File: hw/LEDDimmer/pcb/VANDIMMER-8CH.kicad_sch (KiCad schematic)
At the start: 42 parts, among them J1 PWR_IN, J10 BTN1, J11 BTN2, J2 CH1, J3 CH2, J4 CH3, J5 CH4, J6 CH5, J7 CH6, J8 CH7, J9 CH8, Q1 IRLZ44N, Q2 IRLZ44N, Q3 IRLZ44N, Q4 IRLZ44N, Q5 IRLZ44N, Q6 IRLZ44N, Q7 IRLZ44N, Q8 IRLZ44N, U1 LM1117T-3.3, U2 ESP32-DevkitC-1

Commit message: hw
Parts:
- J2, J3, J4, J5, J6, J7, J8, J9: footprint TerminalBlock:TerminalBlock_bornier-2_P5.08mm -> TerminalBlock:TerminalBlock_Xinya_XY308-2.54-2P_1x02_P2.54mm_Horizontal
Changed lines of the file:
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@@
 			)
 		)
-		(property "Footprint" "TerminalBlock:TerminalBlock_bornier-2_P5.08mm"
+		(property "Footprint" "TerminalBlock:TerminalBlock_Xinya_XY308-2.54-2P_1x02_P2.54mm_Horizontal"
 			(at 148.59 82.55 0)
 			(effects
@@
 			)
 		)
-		(property "Footprint" "TerminalBlock:TerminalBlock_bornier-2_P5.08mm"
+		(property "Footprint" "TerminalBlock:TerminalBlock_Xinya_XY308-2.54-2P_1x02_P2.54mm_Horizontal"
 			(at 189.23 82.55 0)
 			(effects
@@
 			)
 		)
-		(property "Footprint" "TerminalBlock:TerminalBlock_bornier-2_P5.08mm"
+		(property "Footprint" "TerminalBlock:TerminalBlock_Xinya_XY308-2.54-2P_1x02_P2.54mm_Horizontal"
 			(at 229.87 82.55 0)
 			(effects
@@
 			)
 		)
-		(property "Footprint" "TerminalBlock:TerminalBlock_bornier-2_P5.08mm"
+		(property "Footprint" "TerminalBlock:TerminalBlock_Xinya_XY308-2.54-2P_1x02_P2.54mm_Horizontal"
 			(at 270.51 82.55 0)
 			(effects
@@
 			)
 		)
-		(property "Footprint" "TerminalBlock:TerminalBlock_bornier-2_P5.08mm"
+		(property "Footprint" "TerminalBlock:TerminalBlock_Xinya_XY308-2.54-2P_1x02_P2.54mm_Horizontal"
 			(at 152.4 41.91 0)
 			(effects
@@
 			)
 		)
-		(property "Footprint" "TerminalBlock:TerminalBlock_bornier-2_P5.08mm"
+		(property "Footprint" "TerminalBlock:TerminalBlock_Xinya_XY308-2.54-2P_1x02_P2.54mm_Horizontal"
 			(at 193.04 41.91 0)
 			(effects
@@
 			)
 		)
-		(property "Footprint" "TerminalBlock:TerminalBlock_bornier-2_P5.08mm"
+		(property "Footprint" "TerminalBlock:TerminalBlock_Xinya_XY308-2.54-2P_1x02_P2.54mm_Horizontal"
 			(at 233.68 41.91 0)
 			(effects
@@
 			)
 		)
-		(property "Footprint" "TerminalBlock:TerminalBlock_bornier-2_P5.08mm"
+		(property "Footprint" "TerminalBlock:TerminalBlock_Xinya_XY308-2.54-2P_1x02_P2.54mm_Horizontal"
 			(at 274.32 41.91 0)
 			(effects

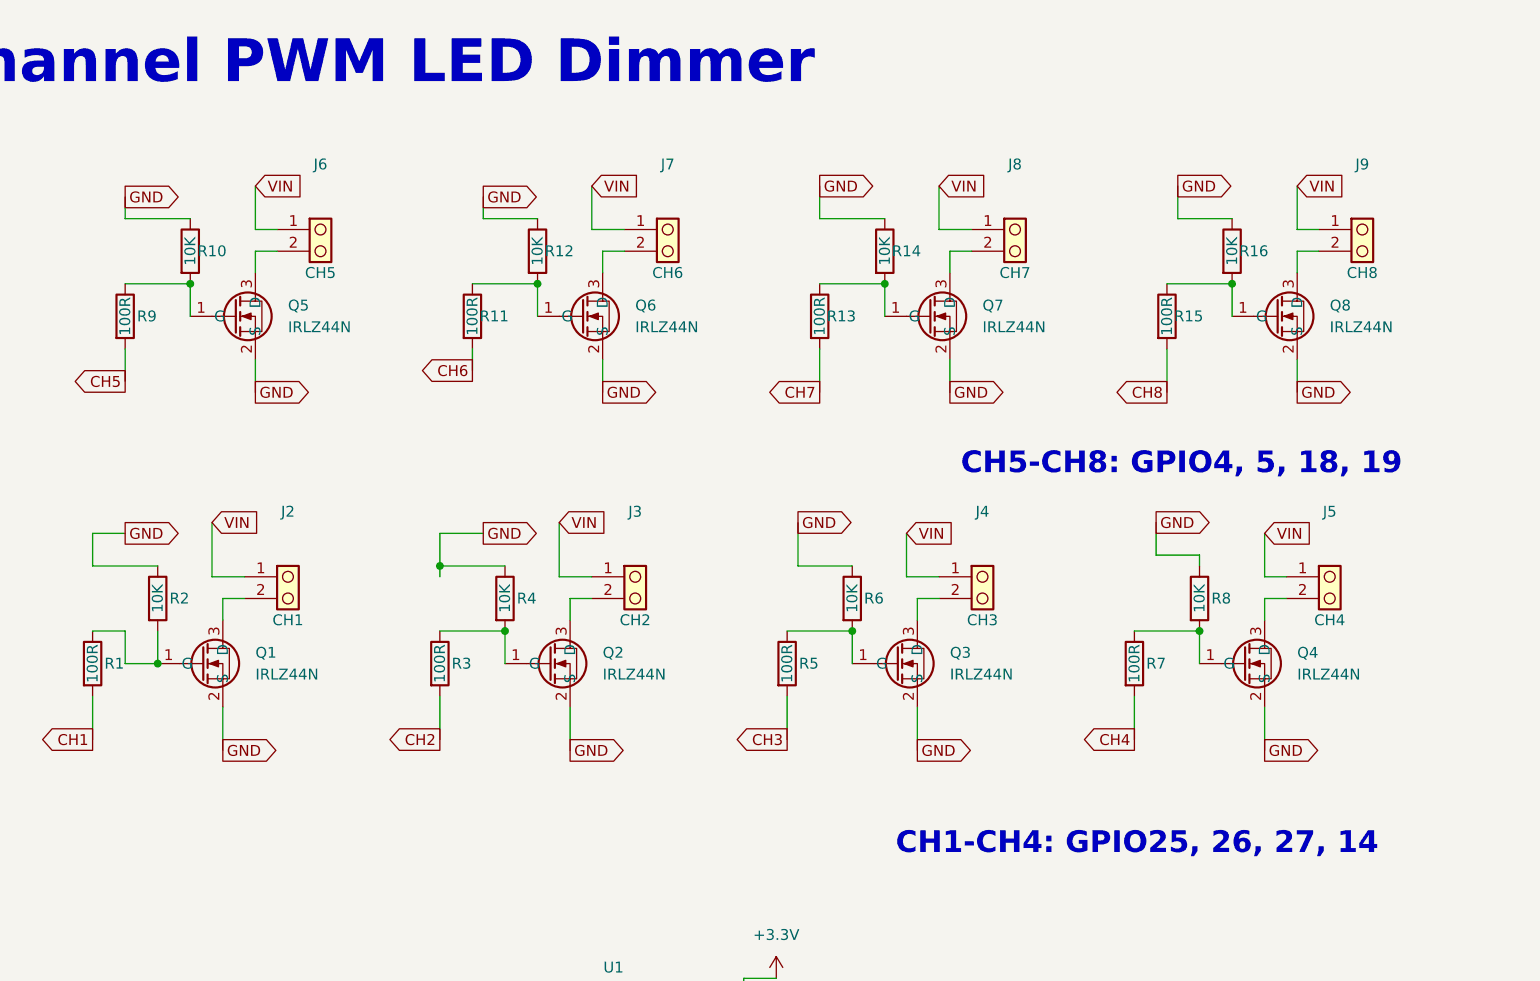
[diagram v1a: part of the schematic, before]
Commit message: v4
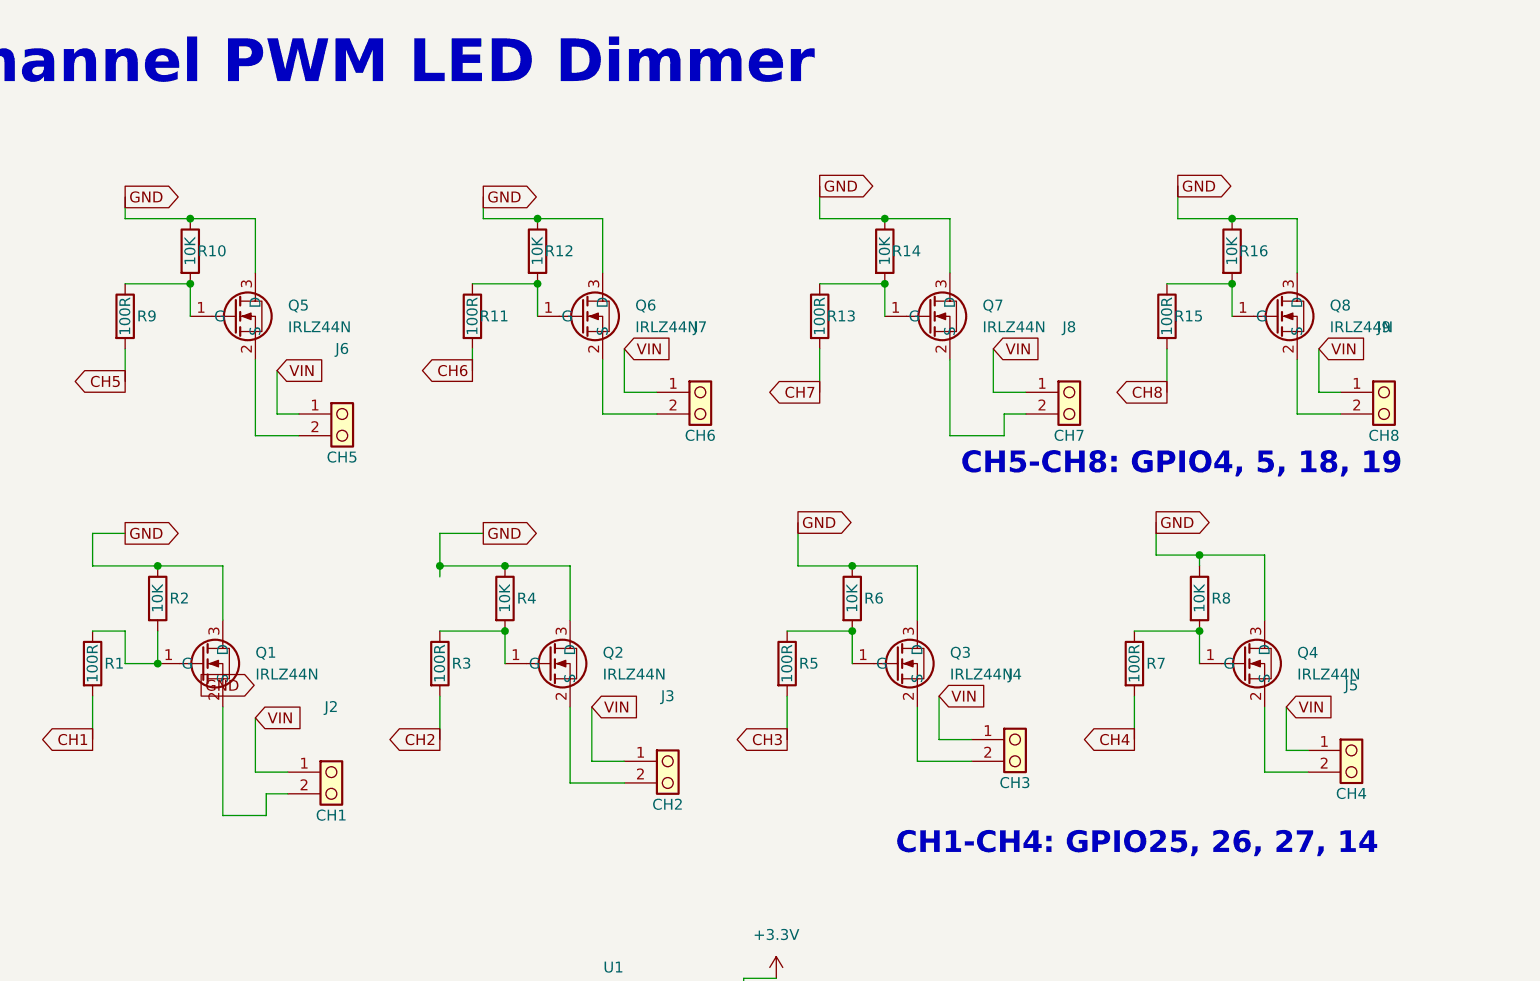
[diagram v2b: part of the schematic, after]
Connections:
- net GND: now also Q1.3 (D), Q2.3 (D), Q3.3 (D), Q4.3 (D), Q5.3 (D), Q6.3 (D), Q7.3 (D), Q8.3 (D); no longer Q1.2 (S), Q2.2 (S), Q3.2 (S), Q4.2 (S), Q5.2 (S), Q6.2 (S), Q7.2 (S), Q8.2 (S)
- net at J2.2 (Pin_2): now also Q1.2 (S); no longer Q1.3 (D)
- net at J3.2 (Pin_2): now also Q2.2 (S); no longer Q2.3 (D)
- net at J4.2 (Pin_2): now also Q3.2 (S); no longer Q3.3 (D)
- net at J5.2 (Pin_2): now also Q4.2 (S); no longer Q4.3 (D)
- net at J6.2 (Pin_2): now also Q5.2 (S); no longer Q5.3 (D)
- net at J7.2 (Pin_2): now also Q6.2 (S); no longer Q6.3 (D)
- net at J8.2 (Pin_2): now also Q7.2 (S); no longer Q7.3 (D)
- net at J9.2 (Pin_2): now also Q8.2 (S); no longer Q8.3 (D)
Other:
- moved on the sheet: J2, J3, J4, J5, J6, J7, J8, J9
